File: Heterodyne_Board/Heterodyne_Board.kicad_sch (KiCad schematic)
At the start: 44 parts, among them J1 AVR-ISP-6, J2 Speaker, SW1 SW_SPST, U1 ATtiny85-20P, U2 TLV9054xD, U3 AP2112K-3.3, U4 LM386, U5 W25X40CLSN, U6 TLV9054xD, U7 TLV9054xD

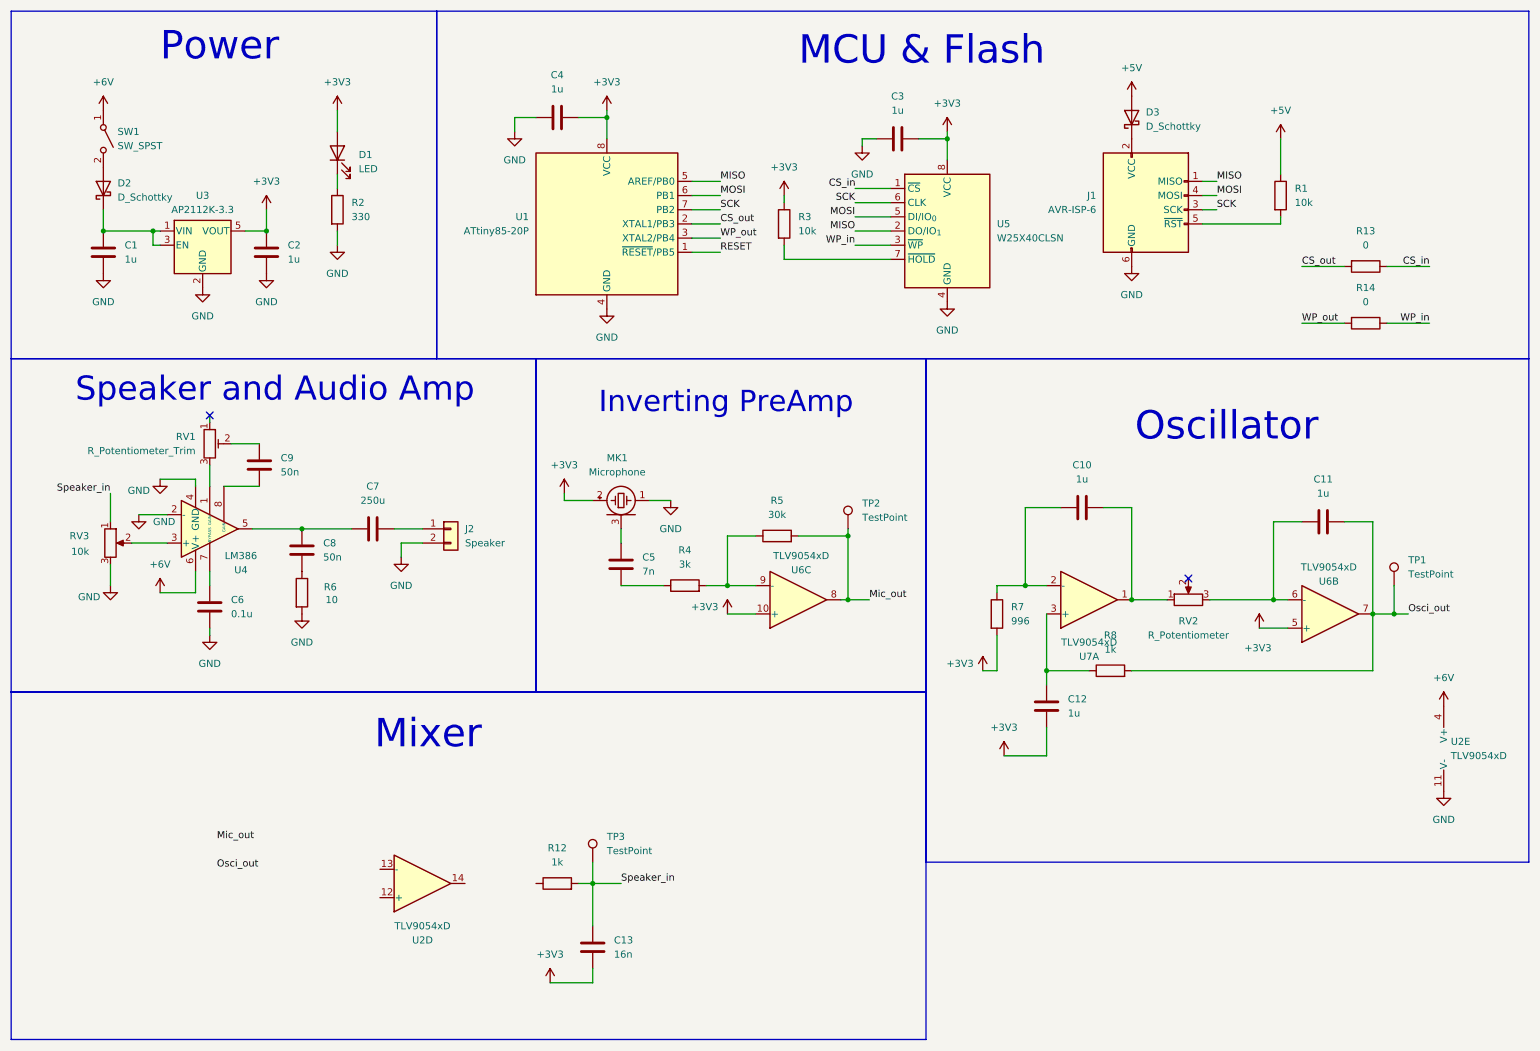
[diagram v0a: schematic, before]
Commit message: fixed osc and mixer
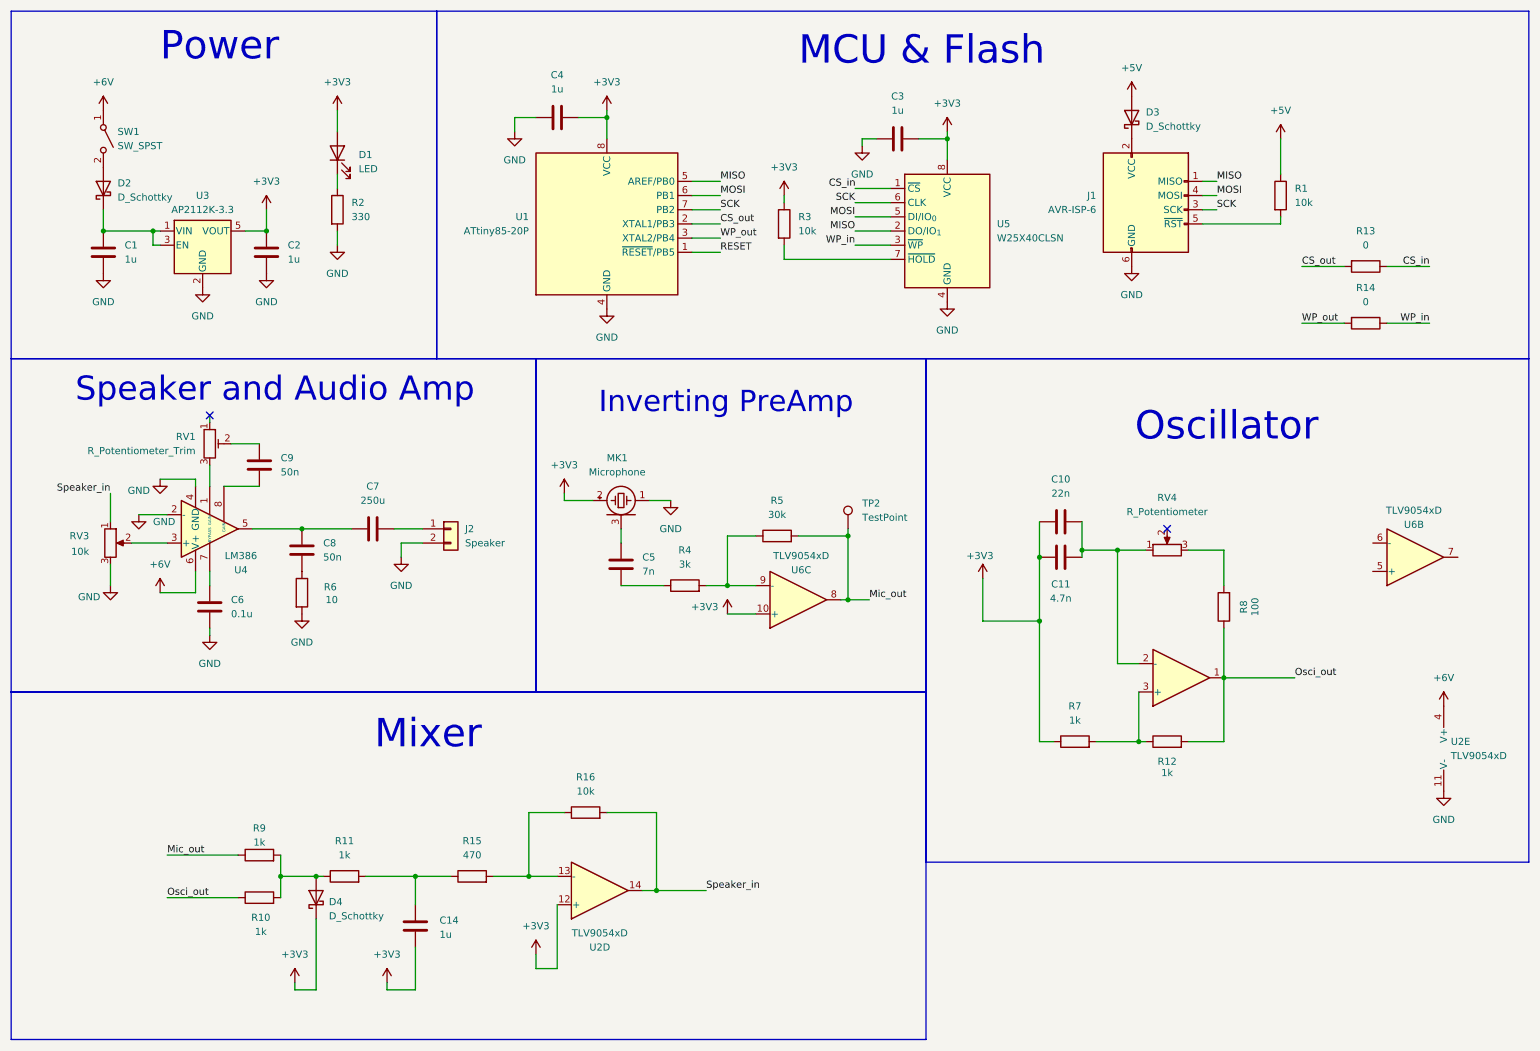
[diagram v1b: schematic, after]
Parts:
- removed C12: 1u, symbol Device:C
- removed C13: 16n, symbol Device:C
- removed RV2: R_Potentiometer, symbol Device:R_Potentiometer
- removed TP1, TP3: TestPoint, symbol Connector:TestPoint
- added C14: 1u, symbol Device:C
- added D4: D_Schottky, symbol Device:D_Schottky
- added R10, R11, R9: 1k, symbol Device:R
- added R15: 470, symbol Device:R
- added R16: 10k, symbol Device:R
- added RV4: R_Potentiometer, symbol Device:R_Potentiometer
- C10: value 1u -> 22n
- C11: value 1u -> 4.7n
- R7: value 996 -> 1k
- R8: value 1k -> 100
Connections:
- net +3V3: now also C10.1, C11.1, R7.1, U2.12 (+), C14.2, D4.1 (K); no longer R7.2, U6.5 (+)
- net Mic_out: now also R9.1
- net Osci_out: now also R12.2, R8.1, U7.1, R10.1; no longer C11.2, R8.2, U6.7
- net Speaker_in: now also U2.14, R16.2; no longer R12.2
- net at C10.2: now also C11.2, U7.2 (-), RV4.1; no longer U7.1
- net at U6.6 (-): no longer C11.1
- net at R12.1: now also R7.2, U7.3 (+)
- net at U2.13 (-): now also R15.2, R16.1
- new net: D4.2 (A), R10.2, R11.1, R9.2
- new net: R8.2, RV4.3
- new net: C14.1, R11.2, R15.1
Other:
- moved on the sheet: U2D, U6B
